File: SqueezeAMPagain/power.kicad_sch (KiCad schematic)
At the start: 63 parts, among them J6 Barrel_Jack_Switch, J7 Conn_01x02_Pin, Q1 Q_NPN_BEC, Q2 AO3401A, Q3 AO3401A, Q4 AO3401A, Q5 Q_NPN_BEC, Q6 AO3401A, Q7 AO3401A, U5 AMS1117-3.3, U6 TPS5430DDA

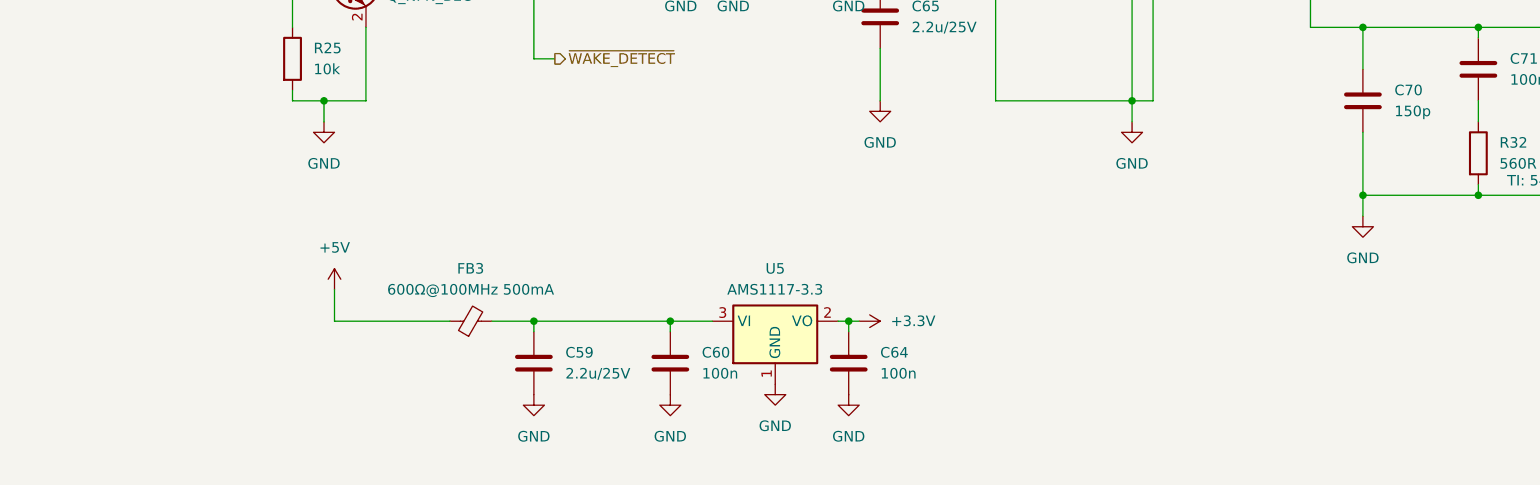
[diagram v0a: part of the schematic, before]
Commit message: Update SqueezeAMPagain.kicad_pcb, SqueezeAMPagain.kicad_prl, SqueezeAMPagain.kicad_pro, and 4 more files
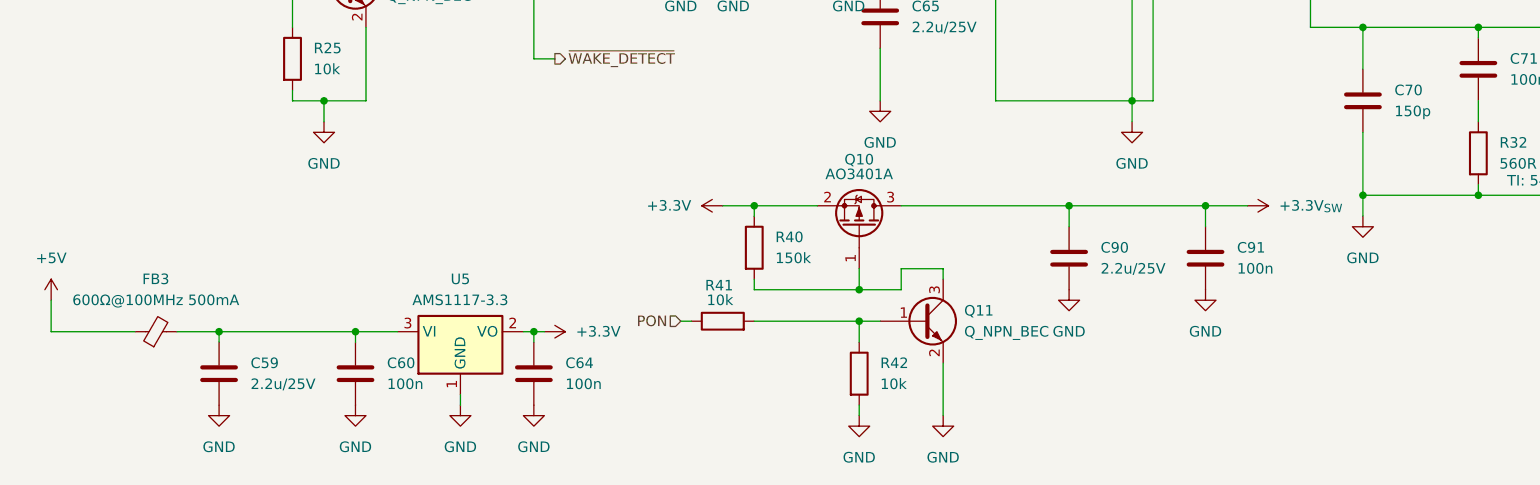
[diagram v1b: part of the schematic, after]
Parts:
- added C90: 2.2u/25V, Capacitor_SMD:C_0805_2012Metric, symbol Device:C
- added C91: 100n, Capacitor_SMD:C_0603_1608Metric, symbol Device:C
- added Q10: AO3401A, Package_TO_SOT_SMD:SOT-23, symbol Transistor_FET:AO3401A
- added Q11: Q_NPN_BEC, Package_TO_SOT_SMD:SOT-23, symbol Device:Q_NPN_BEC
- added R40: 150k, Resistor_SMD:R_0603_1608Metric, symbol Device:R
- added R41, R42: 10k, Resistor_SMD:R_0603_1608Metric, symbol Device:R
- D2: value SS34 550mV 2A -> SS34 550mV 2A
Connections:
- net +3.3V: now also Q10.2 (S), R40.1
- net GND: now also C90.2, C91.2, Q11.2 (E), R42.2
- net PON: now also R41.1
- new net: Q10.1 (G), Q11.3 (C), R40.2
- new net: Q11.1 (B), R41.2, R42.1
- new net +3.3V_{SW}: C90.1, C91.1, Q10.3 (D)
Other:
- moved on the sheet: C59, C60, C64, FB3, U5
